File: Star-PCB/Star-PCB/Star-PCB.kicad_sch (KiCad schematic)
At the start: 6 parts

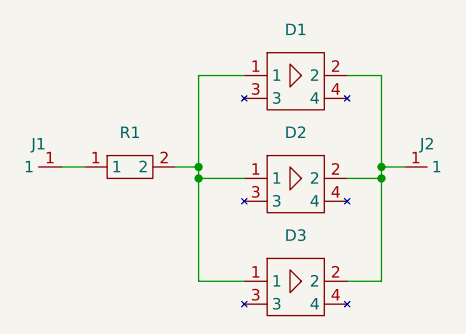
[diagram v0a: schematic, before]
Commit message: Schematics Done
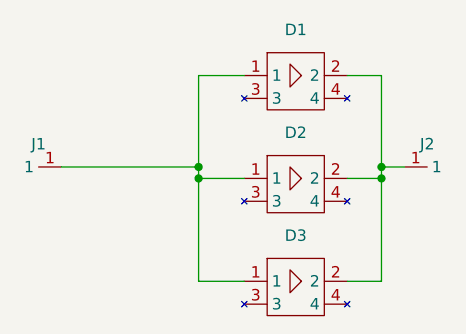
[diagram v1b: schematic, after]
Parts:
- removed R1: ~, Resistor_SMD:R_0201_0603Metric, symbol Star-Library:ERJP03J220V
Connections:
- net at D1.1, D2.1, D3.1: now also J1.1
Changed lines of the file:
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@@
-    (stroke (width 0) (type default))
-  )
-  (wire (pts (xy 107.95 90.17) (xy 110.49 90.17))
     (stroke (width 0) (type default))
   )
@@
     (stroke (width 0) (type default))
   )
-  (wire (pts (xy 95.25 90.17) (xy 97.79 90.17))
+  (wire (pts (xy 95.25 90.17) (xy 110.49 90.17))
     (stroke (width 0) (type default))
   )
@@
         )
       )
-    )
-  )
-  (symbol (lib_id "Star-Library:ERJP03J220V") (at 102.87 90.17 0) (unit 1)
-    (in_bom yes) (on_board yes) (dnp no) (fields_autoplaced)
-    (property "Reference" "R1" (at 102.87 86.36 0)
-      (effects (font (size 1.27 1.27)))
-    )
-    (property "Value" "~" (at 102.87 90.17 0)
-      (effects (font (size 1.27 1.27)))
-    )
-    (property "Footprint" "Resistor_SMD:R_0201_0603Metric" (at 102.87 90.17 0)
-      (effects (font (size 1.27 1.27)) hide)
-    )
-    (property "Datasheet" "" (at 102.87 90.17 0)
-      (effects (font (size 1.27 1.27)) hide)
-    )
-    (pin "1")
-    (pin "2")
-    (instances
-      (project "Star-PCB"
-        (path "/89137b40-bd1a-4b6b-9428-fda32c28674d"
-          (reference "R1") (unit 1)
-        )
-      )
